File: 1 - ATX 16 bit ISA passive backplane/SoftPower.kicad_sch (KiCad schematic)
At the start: 57 parts, among them J18 ATX POWER, SW1 POWER, U1 74HCT14, U2 LM7905, U3 74HCT74

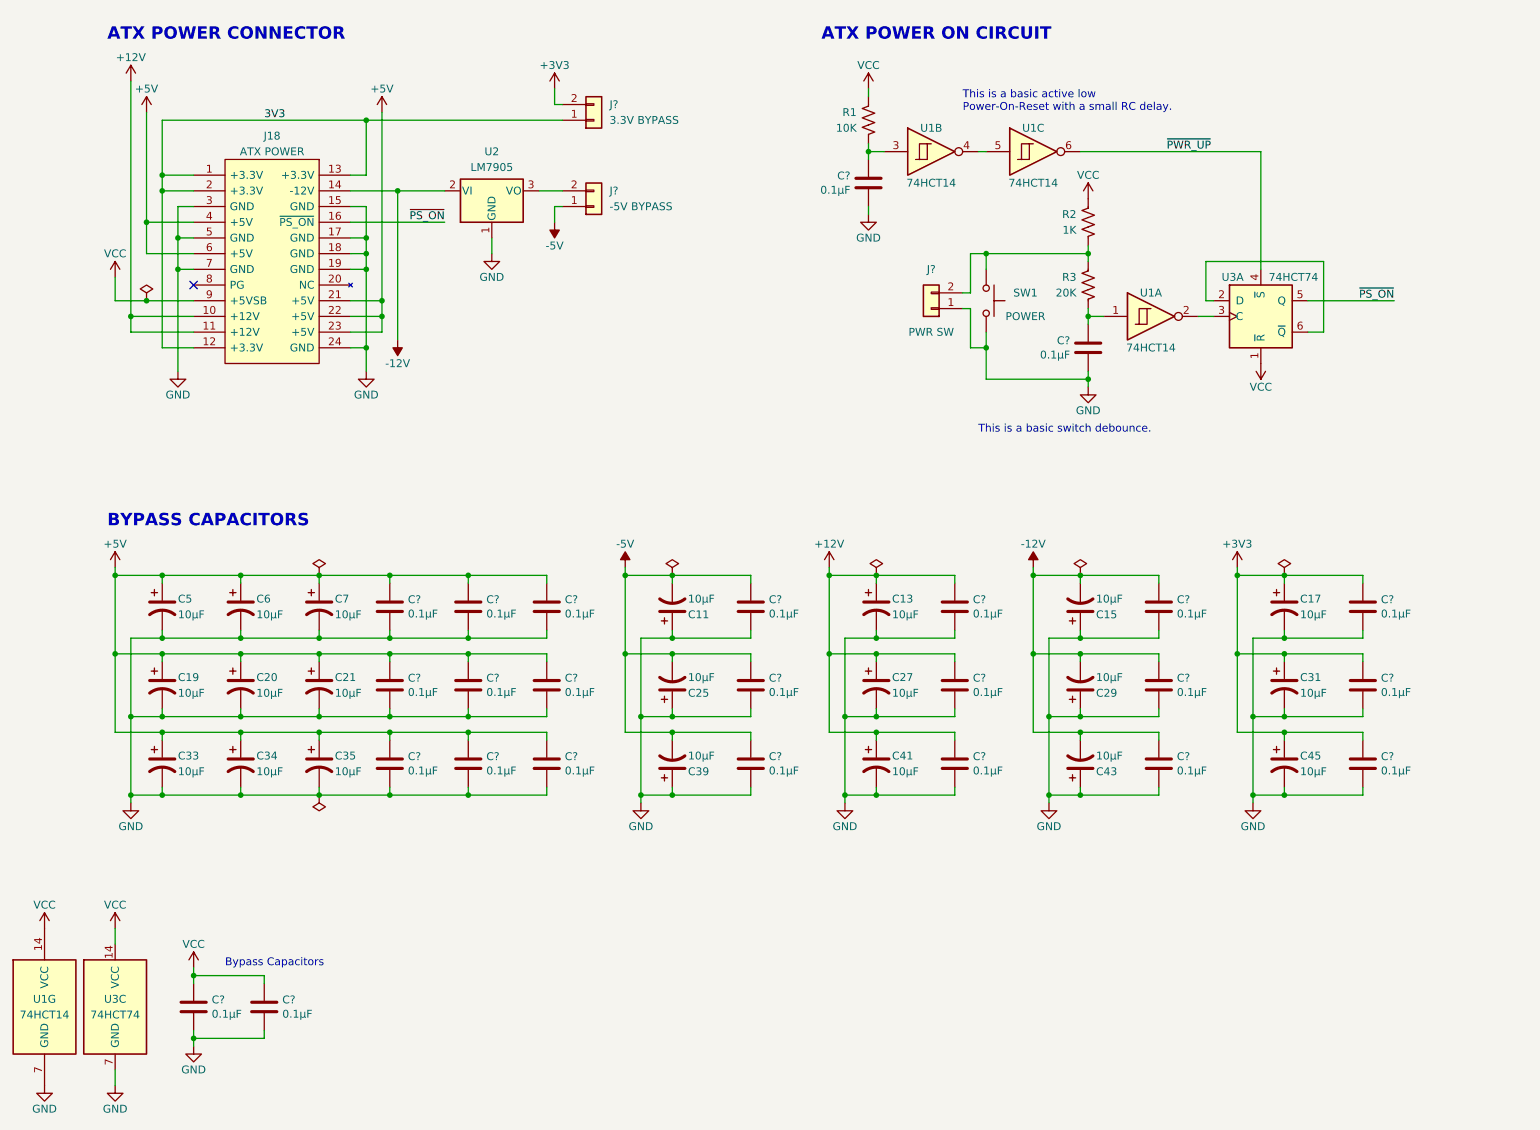
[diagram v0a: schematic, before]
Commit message: Finally finalized the backplane to my liking.
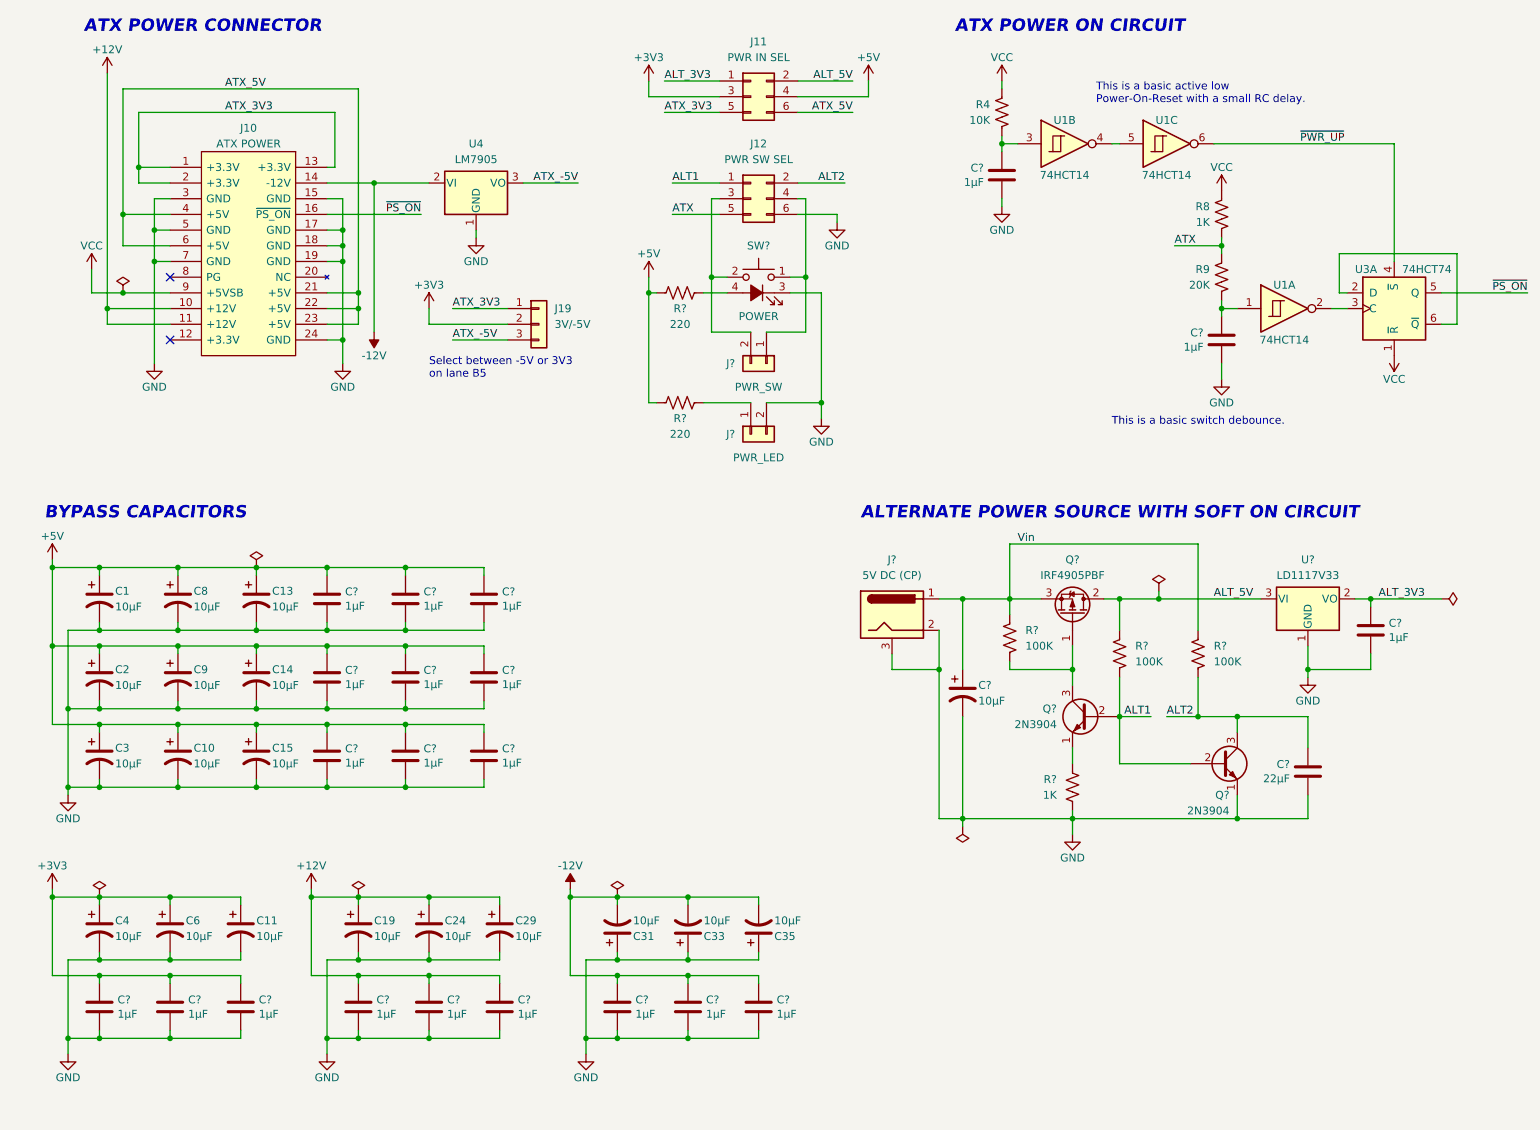
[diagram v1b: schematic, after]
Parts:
- removed C11, C25, C39: 10µF, Capacitor_THT:CP_Radial_D6.3mm_P2.50mm, symbol Device:C_Polarized_US
- removed C? (x5): 0.1µF, Capacitor_THT:C_Disc_D3.0mm_W1.6mm_P2.50mm, symbol Device:C
- removed J?: 3.3V BYPASS, Connector_PinHeader_2.54mm:PinHeader_1x02_P2.54mm_Vertical, symbol Connector_Generic:Conn_01x02
- removed J?: -5V BYPASS, 0_Library:PinHeader_1x2_Vertical (Modified), symbol Connector_Generic:Conn_01x02
- removed J?: PWR SW, 0_Library:PinHeader_1x2_Vertical (Modified), symbol Connector_Generic:Conn_01x02
- removed SW1: POWER, Button_Switch_THT:SW_PUSH-12mm, symbol Switch:SW_Push
- removed unit 7 of U1
- removed U2: LM7905, Package_TO_SOT_THT:TO-220-3_Horizontal_TabDown, symbol Regulator_Linear:LM7905_TO220
- removed unit 3 of U3
- added C?: 10µF, Capacitor_THT:CP_Radial_D6.3mm_P2.50mm, symbol Device:C_Polarized_US
- added C?: 22µF, Capacitor_THT:C_Disc_D3.0mm_W1.6mm_P2.50mm, symbol Device:C
- added C?: 1µF, Capacitor_THT:C_Disc_D3.0mm_W1.6mm_P2.50mm, symbol Device:C
- added J11: PWR IN SEL, Connector_PinHeader_2.54mm:PinHeader_2x03_P2.54mm_Vertical, symbol Connector_Generic:Conn_02x03_Odd_Even
- added J12: PWR SW SEL, Connector_PinHeader_2.54mm:PinHeader_2x03_P2.54mm_Vertical, symbol Connector_Generic:Conn_02x03_Odd_Even
- added J19: 3V/-5V, Connector_PinHeader_2.54mm:PinHeader_1x03_P2.54mm_Vertical, symbol Connector_Generic:Conn_01x03
- added J?: PWR_SW, 0_Library:PinHeader_1x2_Vertical (Modified), symbol Connector_Generic:Conn_01x02
- added J?: PWR_LED, 0_Library:PinHeader_1x2_Vertical (Modified), symbol Connector_Generic:Conn_01x02
- added J?: 5V DC (CP), Connector_BarrelJack:BarrelJack_Horizontal, symbol 0_Library:Barrel_Jack
- added Q? (x2): 2N3904, Package_TO_SOT_THT:TO-92_Inline_Wide, symbol Transistor_BJT:2N3904
- added Q?: IRF4905PBF, Package_TO_SOT_THT:TO-220-3_Horizontal_TabDown, symbol Transistor_FET:IRF4905
- added R? (x2): 220, Resistor_THT:R_Axial_DIN0207_L6.3mm_D2.5mm_P10.16mm_Horizontal, symbol Device:R_US
- added R?: 1K, Resistor_THT:R_Axial_DIN0207_L6.3mm_D2.5mm_P10.16mm_Horizontal, symbol Device:R_US
- added R? (x3): 100K, Resistor_THT:R_Axial_DIN0207_L6.3mm_D2.5mm_P10.16mm_Horizontal, symbol Device:R_US
- added SW?: POWER, 0_Library:Pushbutton_12mm_LED, symbol Switch:SW_Push_LED
- added U4: LM7905, Package_TO_SOT_THT:TO-220-3_Horizontal_TabDown, symbol Regulator_Linear:L7905
- added U?: LD1117V33, Package_TO_SOT_THT:TO-220-3_Horizontal_TabDown, symbol 0_Library:LM1117-3.3
- C? (x20): value 0.1µF -> 1µF
- renumbered C5 to C1, C34 to C10, C45 to C11, C7 to C13, C21 to C14, C35 to C15, C13 to C19, C19 to C2, C27 to C24, C41 to C29, C33 to C3, C15 to C31, C29 to C33, C43 to C35, C17 to C4, C31 to C6, C6 to C8, C20 to C9, J18 to J10, R1 to R4, R2 to R8, R3 to R9
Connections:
- net +3V3: now also J11.3 (Pin_3), J19.2 (Pin_2)
- net +5V: now also J11.4 (Pin_4), R?.2, R?.2; no longer J10.21 (+5V), J10.22 (+5V), J10.23 (+5V), J10.4 (+5V), J10.6 (+5V)
- net -12V: now also U4.2 (VI)
- net GND: now also C?.2, C?.2, C?.2, J12.6 (Pin_6), J?.2, J?.2 (Pin_2), J?.3, Q?.1 (E), R?.1, SW?.3 (K), U4.1 (GND), U?.1 (GND)
- net ATX: now reaches R8.2, R9.1
- net ATX: now also J12.5 (Pin_5)
- net 3V3 renamed ATX_3V3
- net ATX_3V3: now also J11.5 (Pin_5), J19.1 (Pin_1); no longer J10.12 (+3.3V)
- new net: J12.4 (Pin_4), J?.1 (Pin_1), SW?.1
- new net: J12.3 (Pin_3), J?.2 (Pin_2), SW?.2
- new net: Q?.1 (E), R?.2
- new net: Q?.1 (G), Q?.3 (C), R?.1
- new net: R?.1, SW?.4 (A)
- new net: J?.1 (Pin_1), R?.1
- new net ALT1: J12.1 (Pin_1), Q?.2 (B), Q?.2 (B), R?.1
- new net ALT2: C?.1, J12.2 (Pin_2), Q?.3 (C), R?.1
- new net ALT_3V3: C?.1, J11.1 (Pin_1), U?.2 (VO)
- new net ALT_5V: J11.2 (Pin_2), Q?.2 (D), R?.2, U?.3 (VI)
- new net ATX_-5V: J19.3 (Pin_3), U4.3 (VO)
- new net ATX_5V: J10.21 (+5V), J10.22 (+5V), J10.23 (+5V), J10.4 (+5V), J10.6 (+5V), J11.6 (Pin_6)
- new net Vin: C?.1, J?.1, Q?.3 (S), R?.2, R?.2
- no-connect marks 1 -> 2
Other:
- note added: "ALTERNATE POWER SOURCE WITH SOFT ON CIRCUIT"
- note added: "Select between -5V or 3V3 on lane B5"
- note removed: "Bypass Capacitors"
- moved on the sheet: C1, C10, C11, C13, C14, C15, C19, C2, C24, C29, C3, C31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
